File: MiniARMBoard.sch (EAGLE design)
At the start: 39 parts, among them CN1 J_USB_MICROAB_HIROSE_ZX62-AB-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, U1 LPC1549JBD48, U2 TPD4S014DSQR, U3 MCP1700T-33, U4 ADR5041, U5 FT234XD-R, X1 FA238V

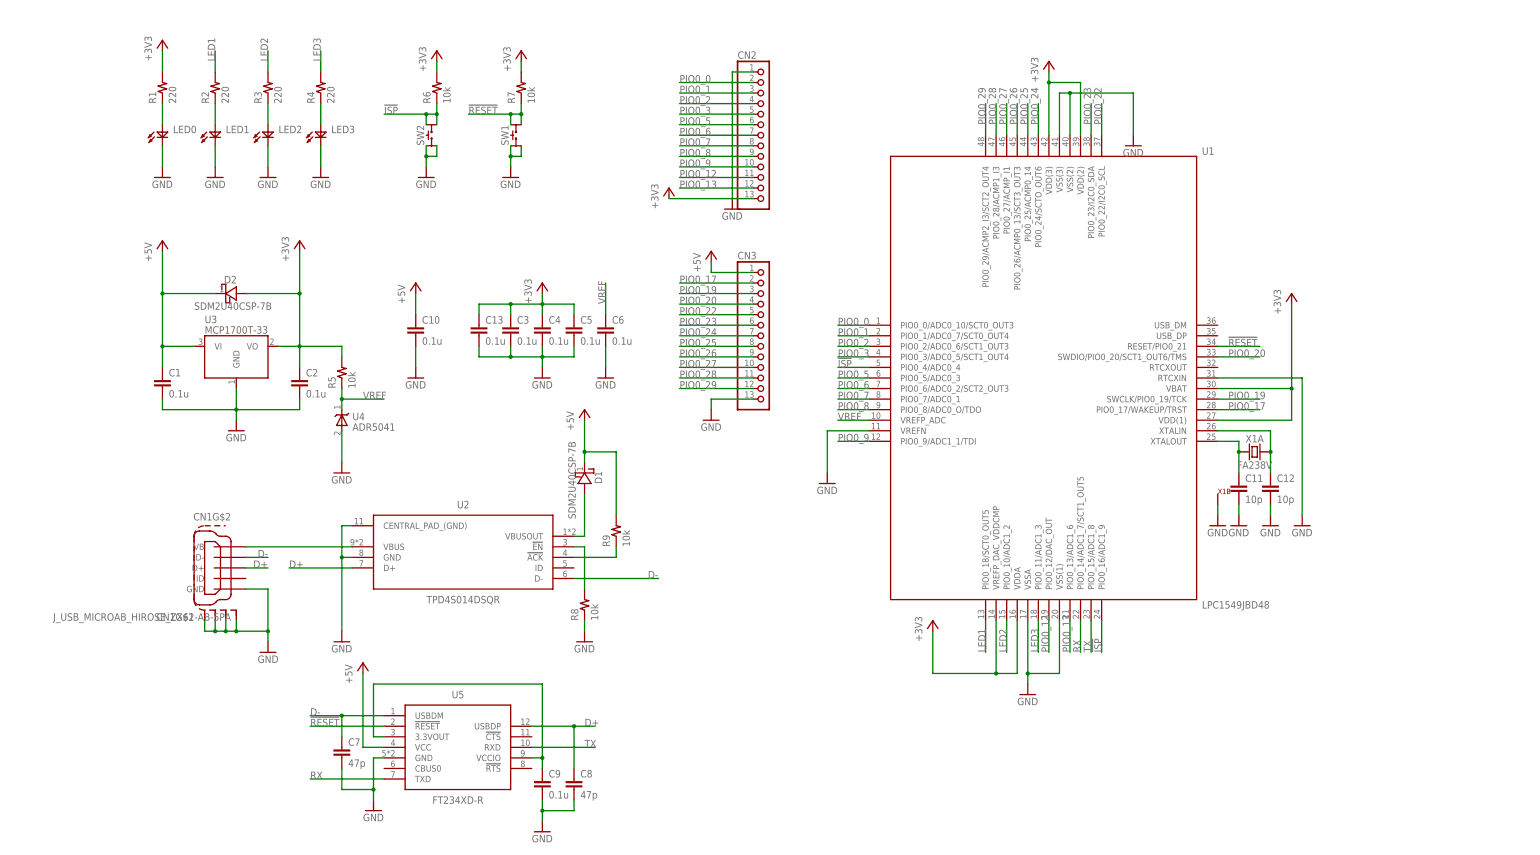
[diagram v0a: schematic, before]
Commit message: 回路図の見た目を整えてみた
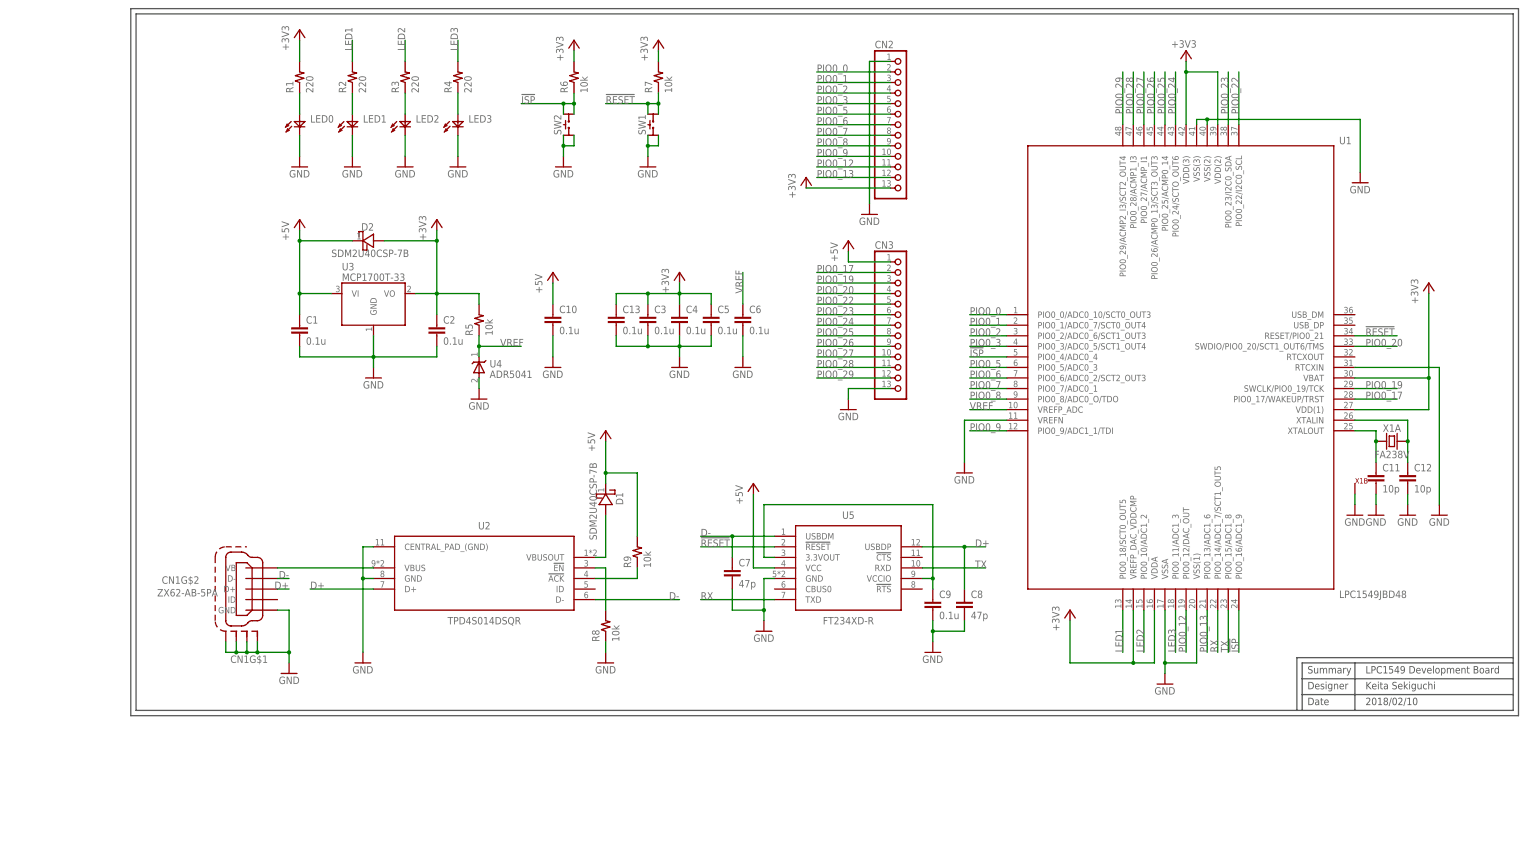
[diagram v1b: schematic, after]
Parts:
- CN1: value J_USB_MICROAB_HIROSE_ZX62-AB-5PA -> ZX62-AB-5PA
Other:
- note added: "2018/02/10"
- note added: "Date"
- note added: "Designer"
- note added: "Keita Sekiguchi"
- note added: "LPC1549 Development Board"
- note added: "Summary"
- moved on the sheet: C1, C10, C11, C12, C13, C2, C3, C4, C5, C6, C7, C8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
